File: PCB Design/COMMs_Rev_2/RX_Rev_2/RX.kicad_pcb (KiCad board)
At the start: 2 copper layers, 40 x 65 mm, 51 parts, among them J1 Conn_01x24_Pin, J2 Conn_01x24_Pin, J3 Conn_01x03_Pin, J4 Conn_01x04_Pin, J5 Conn_01x02_Pin, U1 TLV9101IDCKR, U2 TPD2E007DCKR, U3 INA828IDR, U4 OPA2322AIDGKR

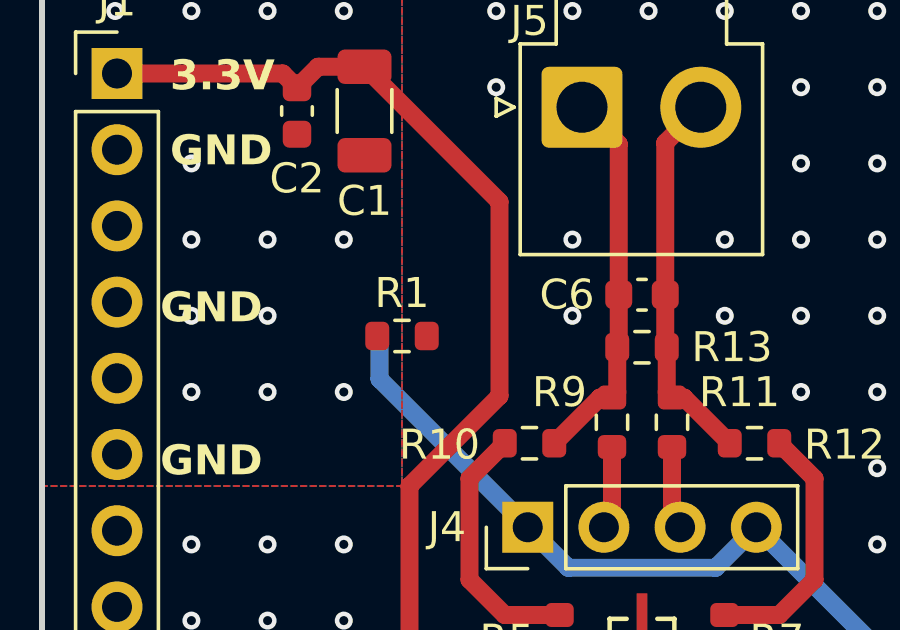
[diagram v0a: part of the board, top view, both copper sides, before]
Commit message: Updated
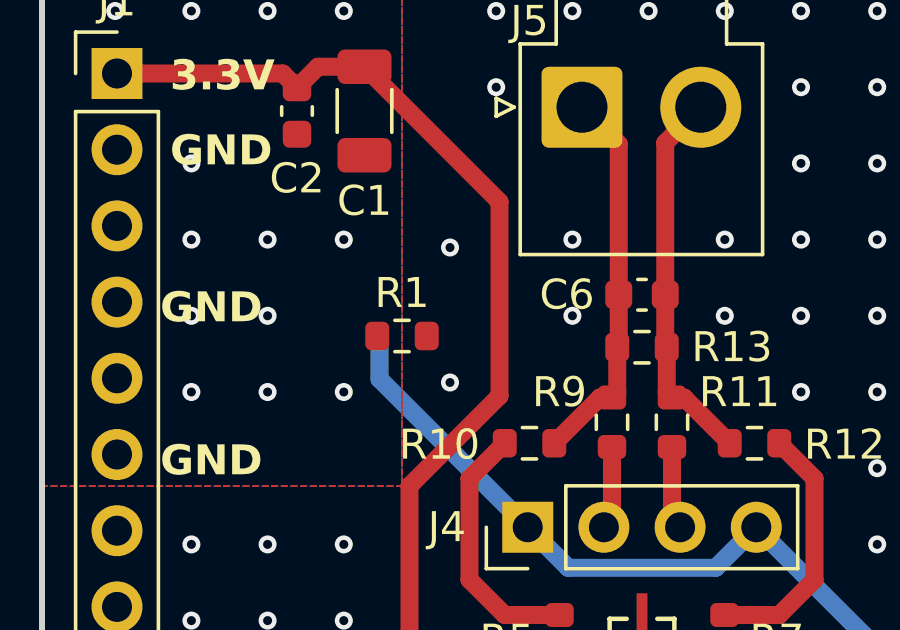
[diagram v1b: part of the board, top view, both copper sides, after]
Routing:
- net AGND: vias 181 -> 183

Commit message: Revert "Updated"
This reverts commit 89be44ed720659141c8ee702c54a520a60db740f.
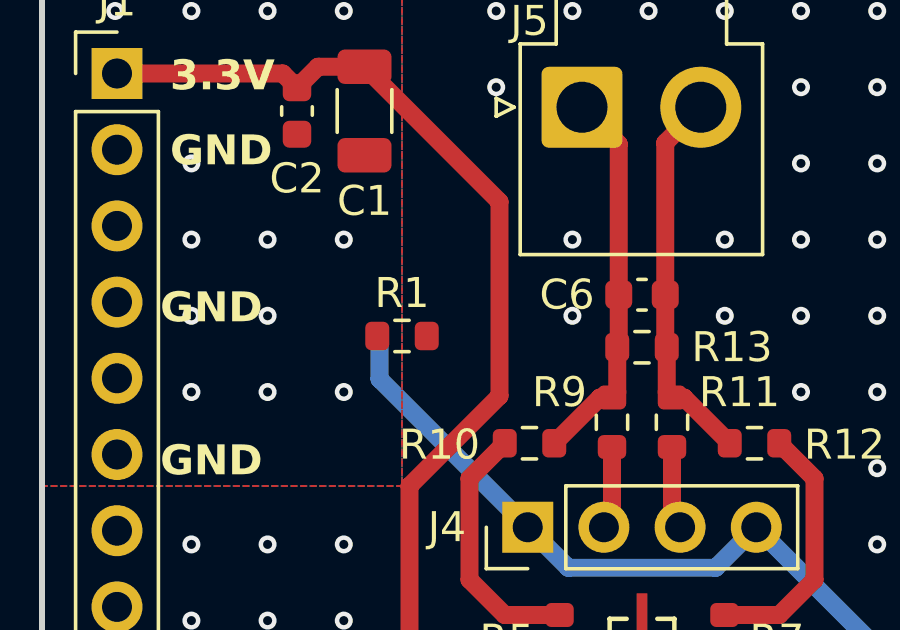
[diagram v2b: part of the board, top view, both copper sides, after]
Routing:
- net AGND: vias 183 -> 181
